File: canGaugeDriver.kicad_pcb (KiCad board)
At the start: 2 copper layers, 74.7 x 41.4 mm, 39 parts, among them J1 CANbed 1.0 Interface, J2 VIN INTERFACE, J3 348260240, U1 TPL7407LA, U2 TPL7407LA

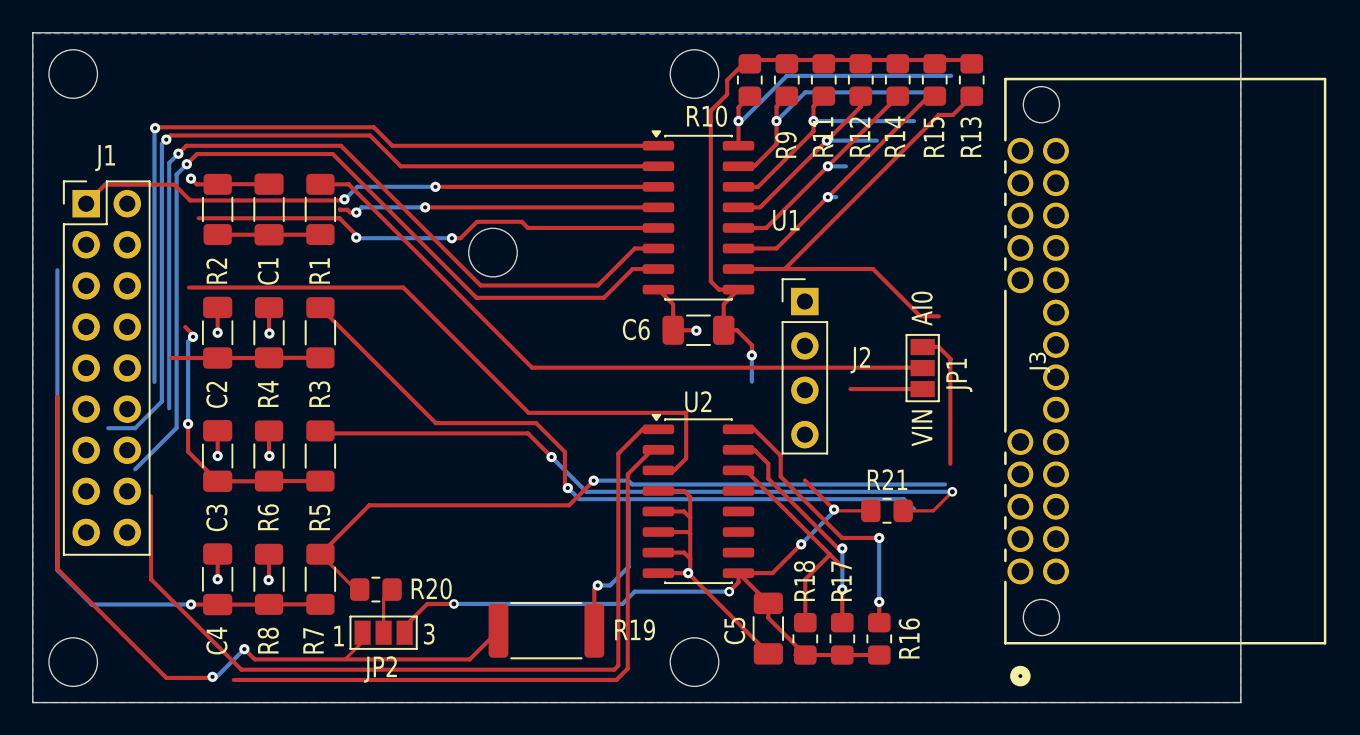
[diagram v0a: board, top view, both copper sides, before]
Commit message: progress
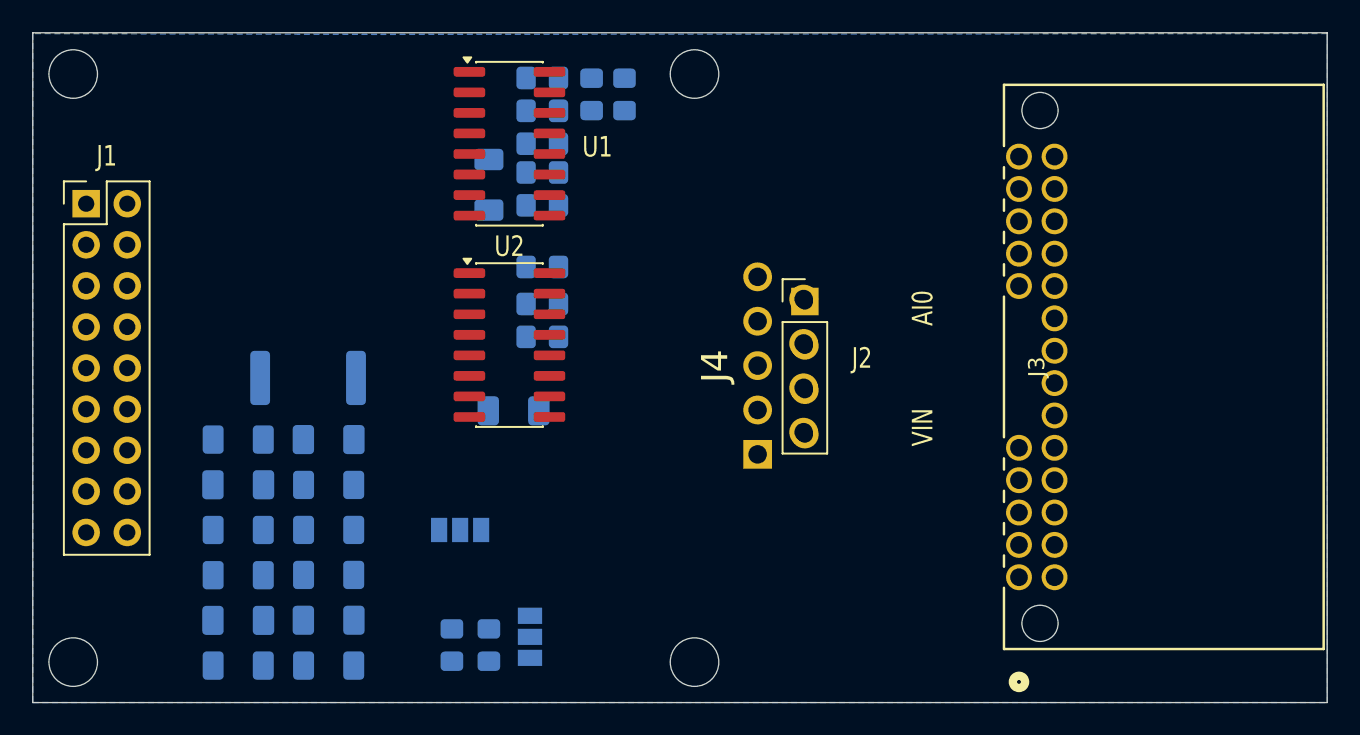
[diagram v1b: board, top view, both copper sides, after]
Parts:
- removed the ? at (130.0, 73.9)
- added J4: DB9'MEAL', canGaugeDriver:DB9-MEAL, F.Cu at (147.8, 80.9)
- C1, C2, C3, C4, C5, C6, JP1, JP2, R1, R10, R11, R12, R13, R14, R15, R16, R17, R18, R19, R2, R20, R21, R3, R4, R5, R6, R7, R8, R9: moved to B.Cu
- moved R16 31.0 mm to (133.1, 74.8), turned to 0 degrees
- moved JP1 30.3 mm to (128.0, 91.1), turned to 180 degrees
- moved R21 28.1 mm to (127.5, 98.2), turned to 90 degrees
- moved R17 27.8 mm to (133.1, 77.1), turned to 0 degrees
- moved R13 27.7 mm to (133.1, 71.0), turned to 0 degrees
- moved R15 24.9 mm to (133.1, 69.0), turned to 0 degrees
- moved R18 24.8 mm to (133.1, 79.1), turned to 0 degrees
- moved R14 22.3 mm to (133.1, 67.2), turned to 0 degrees
- moved R19 21.5 mm to (118.6, 81.7), turned to 0 degrees
- moved C5 20.7 mm to (131.3, 83.7), turned to 180 degrees
- moved R1 19.8 mm to (119.9, 91.1), turned to 180 degrees
- moved R12 19.8 mm to (133.1, 65.2), turned to 0 degrees
- moved R2 18.4 mm to (119.9, 88.3), turned to 0 degrees
- moved C6 15.8 mm to (129.8, 69.7), turned to 90 degrees
- moved U2 15.2 mm to (131.1, 79.6)
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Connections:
- J3 pad 1: unconnected-(J3-Pad1) -> /5V
- J3 pad 10: unconnected-(J3-Pad10) -> /VIN
- J3 pad 11: unconnected-(J3-Pad11) -> GND
- J3 pad 12: unconnected-(J3-Pad12) -> GND
- J3 pad 2: unconnected-(J3-Pad2) -> /5V
- J3 pad 24: unconnected-(J3-Pad24) -> GND
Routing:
- net /VIN: track 87.9 -> 0.00 mm, vias 5 -> 0
- net /D9_FUEL: track 54.0 -> 0.00 mm, vias 1 -> 0
- net /D10_OIL: track 52.6 -> 0.00 mm
- net /AI1: track 52.5 -> 0.00 mm, vias 2 -> 0
- net /D3_SPEED: track 51.6 -> 0.00 mm, vias 1 -> 0
- net /D8_SEATBELT: track 50.4 -> 0.00 mm, vias 1 -> 0
- net /D2_SRS: track 47.3 -> 0.00 mm, vias 1 -> 0
- net /5V: track 44.9 -> 0.00 mm, vias 2 -> 0
- net /AI2: track 43.9 -> 0.00 mm, vias 2 -> 0
- net /AI3: track 43.9 -> 0.00 mm, vias 1 -> 0
- net /AI0_SW: track 41.8 -> 0.00 mm
- net GND: track 40.8 -> 0.00 mm, vias 9 -> 0
- net /D11_TACH: track 38.8 -> 0.00 mm
- net /D12_ALT: track 38.8 -> 0.00 mm
- net /D4_CEL: track 36.7 -> 0.00 mm, vias 2 -> 0
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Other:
- board size 74.7 x 41.4 mm -> 80 x 41.4 mm
